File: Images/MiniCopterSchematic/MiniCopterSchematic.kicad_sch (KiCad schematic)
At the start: 21 parts, among them M1 MOTOR_DC_1, M2 MOTOR_DC_2, M3 MOTOR_DC_3, M4 MOTOR_DC_4, Q1 FQP20NO6L, Q2 FQP20NO6L, Q3 FQP20NO6L, Q4 FQP20NO6L

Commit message: Working on PCB
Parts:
- H1, H2, H3, H4: footprint MountingHole:MountingHole_3.2mm_M3 -> MountingHole:MountingHole_3.2mm_M3_Pad
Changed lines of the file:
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@@
       (effects (font (size 1.27 1.27)) (justify left))
     )
-    (property "Footprint" "MountingHole:MountingHole_3.2mm_M3" (id 2) (at 195.58 54.61 0)
+    (property "Footprint" "MountingHole:MountingHole_3.2mm_M3_Pad" (id 2) (at 195.58 54.61 0)
       (effects (font (size 1.27 1.27)) hide)
     )
@@
       (effects (font (size 1.27 1.27)) (justify left))
     )
-    (property "Footprint" "MountingHole:MountingHole_3.2mm_M3" (id 2) (at 215.9 48.26 0)
+    (property "Footprint" "MountingHole:MountingHole_3.2mm_M3_Pad" (id 2) (at 215.9 48.26 0)
       (effects (font (size 1.27 1.27)) hide)
     )
@@
       (effects (font (size 1.27 1.27)) (justify left))
     )
-    (property "Footprint" "MountingHole:MountingHole_3.2mm_M3" (id 2) (at 215.9 54.61 0)
+    (property "Footprint" "MountingHole:MountingHole_3.2mm_M3_Pad" (id 2) (at 215.9 54.61 0)
       (effects (font (size 1.27 1.27)) hide)
     )
@@
       (effects (font (size 1.27 1.27)) (justify left))
     )
-    (property "Footprint" "MountingHole:MountingHole_3.2mm_M3" (id 2) (at 195.58 48.26 0)
+    (property "Footprint" "MountingHole:MountingHole_3.2mm_M3_Pad" (id 2) (at 195.58 48.26 0)
       (effects (font (size 1.27 1.27)) hide)
     )
@@
     )
     (path "/ac3fbe0c-87a2-45f4-91c1-950d582b1ab5"
-      (reference "H1") (unit 1) (value "MountingHole") (footprint "MountingHole:MountingHole_3.2mm_M3")
+      (reference "H1") (unit 1) (value "MountingHole") (footprint "MountingHole:MountingHole_3.2mm_M3_Pad")
     )
     (path "/67f46d13-4b6b-40ba-b0e1-7fc723cd9aaf"
-      (reference "H2") (unit 1) (value "MountingHole") (footprint "MountingHole:MountingHole_3.2mm_M3")
+      (reference "H2") (unit 1) (value "MountingHole") (footprint "MountingHole:MountingHole_3.2mm_M3_Pad")
     )
     (path "/922275fa-02a3-4b78-8aea-5b6156f8eb65"
-      (reference "H3") (unit 1) (value "MountingHole") (footprint "MountingHole:MountingHole_3.2mm_M3")
+      (reference "H3") (unit 1) (value "MountingHole") (footprint "MountingHole:MountingHole_3.2mm_M3_Pad")
     )
     (path "/9d900d38-a2c3-410e-803b-0eabd5854bf5"
-      (reference "H4") (unit 1) (value "MountingHole") (footprint "MountingHole:MountingHole_3.2mm_M3")
+      (reference "H4") (unit 1) (value "MountingHole") (footprint "MountingHole:MountingHole_3.2mm_M3_Pad")
     )
     (path "/70fbff7a-f0df-40b1-9155-b6abad2a2d0f"

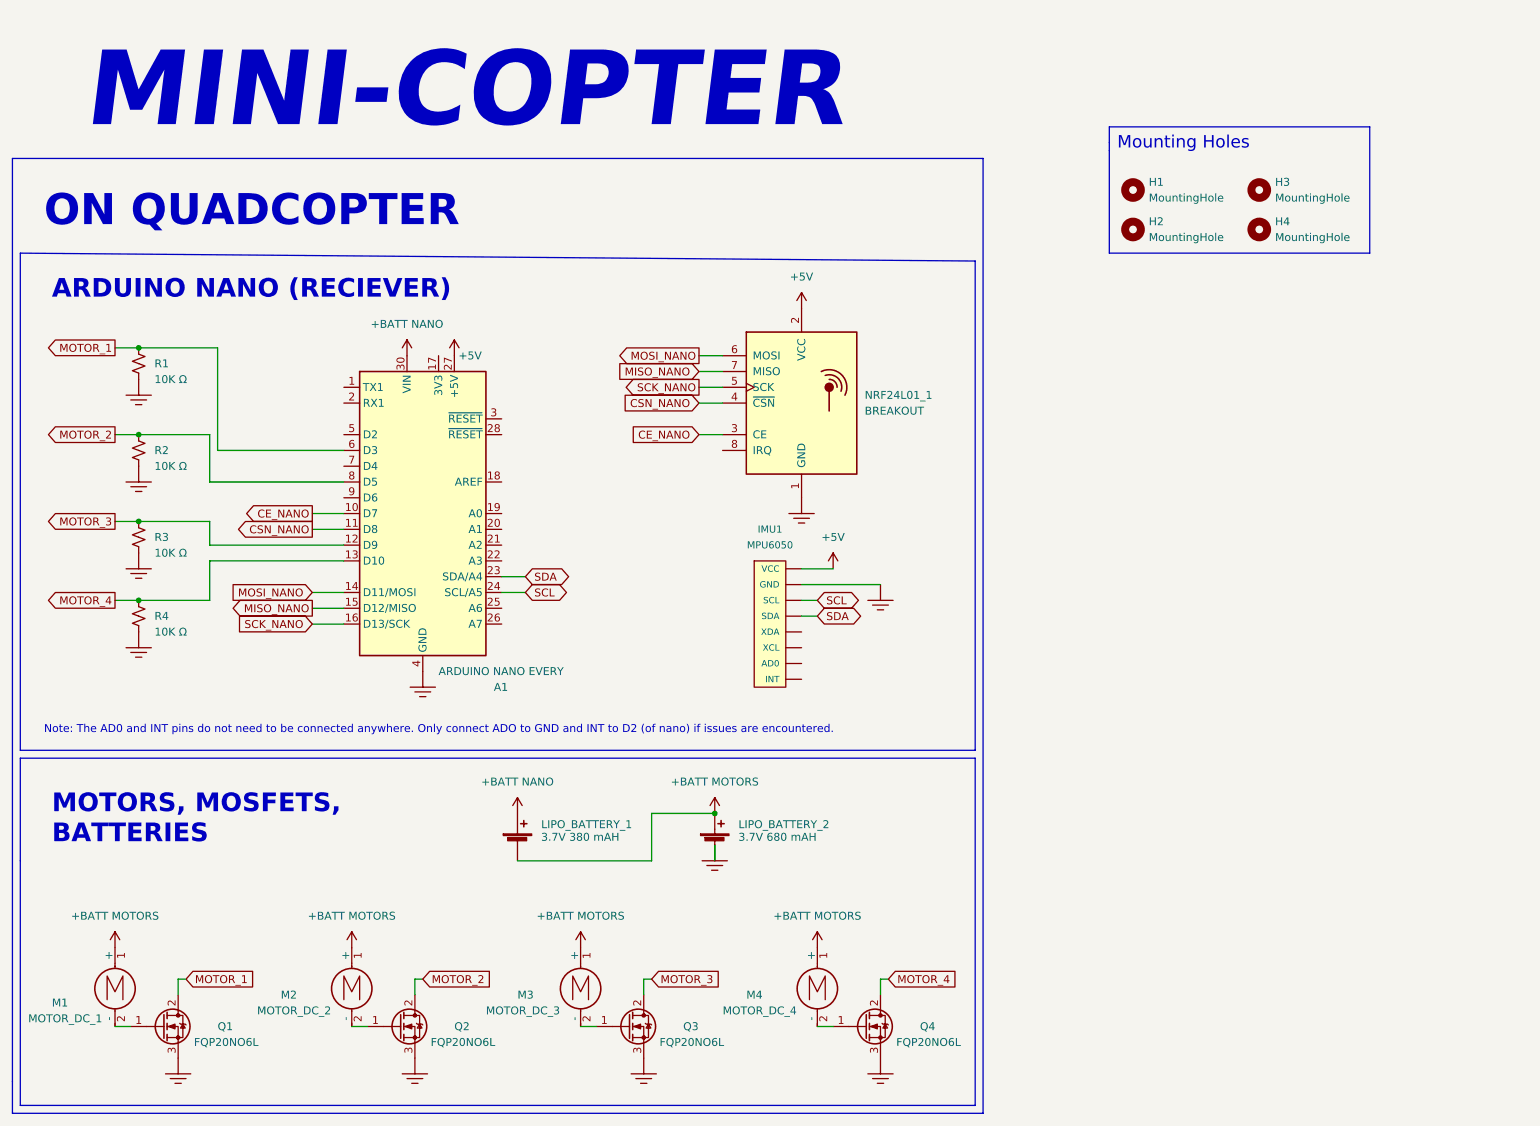
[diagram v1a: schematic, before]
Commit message: Working on PCB organizing and putting on text
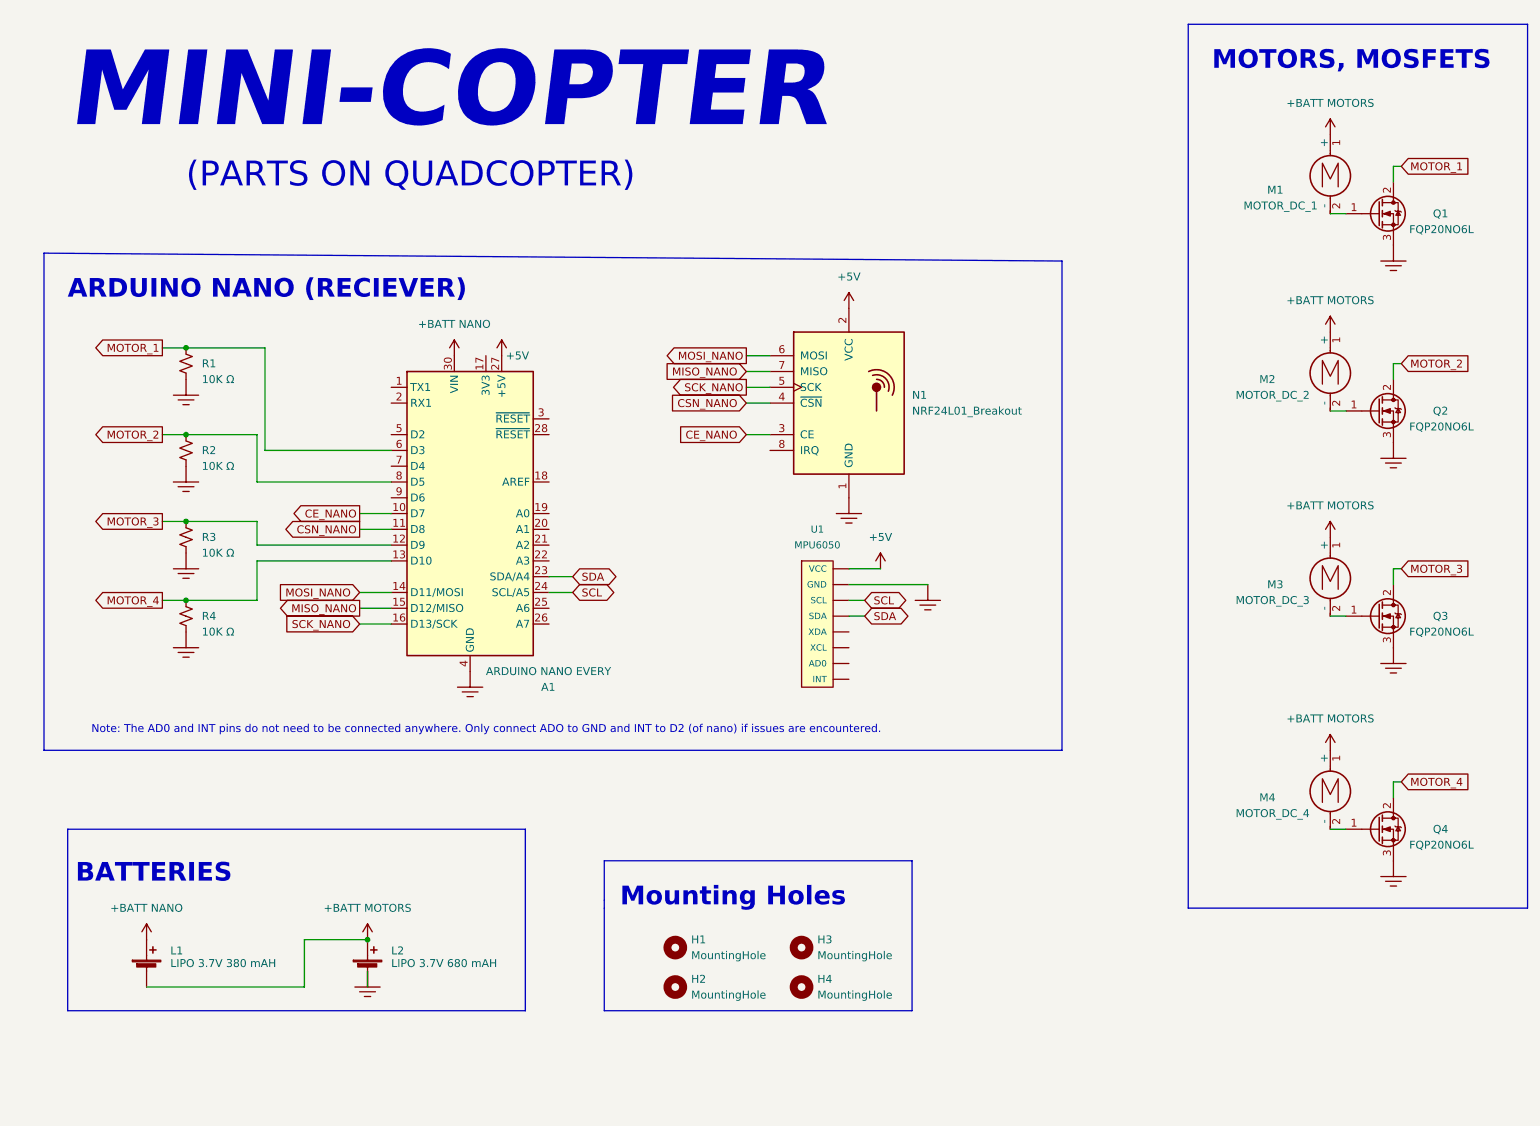
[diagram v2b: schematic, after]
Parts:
- L1: renamed from LIPO_BATTERY_1; value 3.7V 380 mAH -> LIPO 3.7V 380 mAH
- L2: renamed from LIPO_BATTERY_2; value 3.7V 680 mAH -> LIPO 3.7V 680 mAH
- M1, M2, M3, M4: footprint AA_Custom_Components:PowerPad_Pair_4.0x4.0mm -> AA_Custom_Components:PowerPad_Pair_3.0x3.0mm
- N1: renamed from NRF24L01_1; value BREAKOUT -> NRF24L01_Breakout
- renumbered IMU1 to U1
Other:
- note added: "(PARTS ON QUADCOPTER)"
- note added: "BATTERIES"
- note added: "MOTORS, MOSFETS"
- note removed: "MOTORS, MOSFETS, BATTERIES"
- note removed: "ON QUADCOPTER"
- moved on the sheet: A1, H1, H2, H3, H4, L1, L2, M1, M2, M3, M4, N1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
